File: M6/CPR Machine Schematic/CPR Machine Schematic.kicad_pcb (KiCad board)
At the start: 2 copper layers, 134 x 94 mm, 67 parts, among them J1 Contactor 22.2V IN, J10 Stop Button Port, J11 Go Button Port, J12 I2C Port, J13 Raspberry_Pi_2_3, J2 5V Spare Headers, J3 Power Switch, J4 3V3 Spare Headers, J5 12 Spare headers, J6 Battery Spare headers, J7 GND Spare Headers, J8 Force Sensor, J9 Laser Port, Q1 2N3904, Q2 DMG2305UX-13 MOSFET, Q3 FDMS8350LET40, Q4 DMMT5401 PNP, Q6 FDMS8350LET40, Q7 FDMS8350LET40, U1 LT1765EFE-5_PBF, U2 MAX42402AFLB+, U3 MCP6001R, U4 12V Buck, U6 3.3V Buck

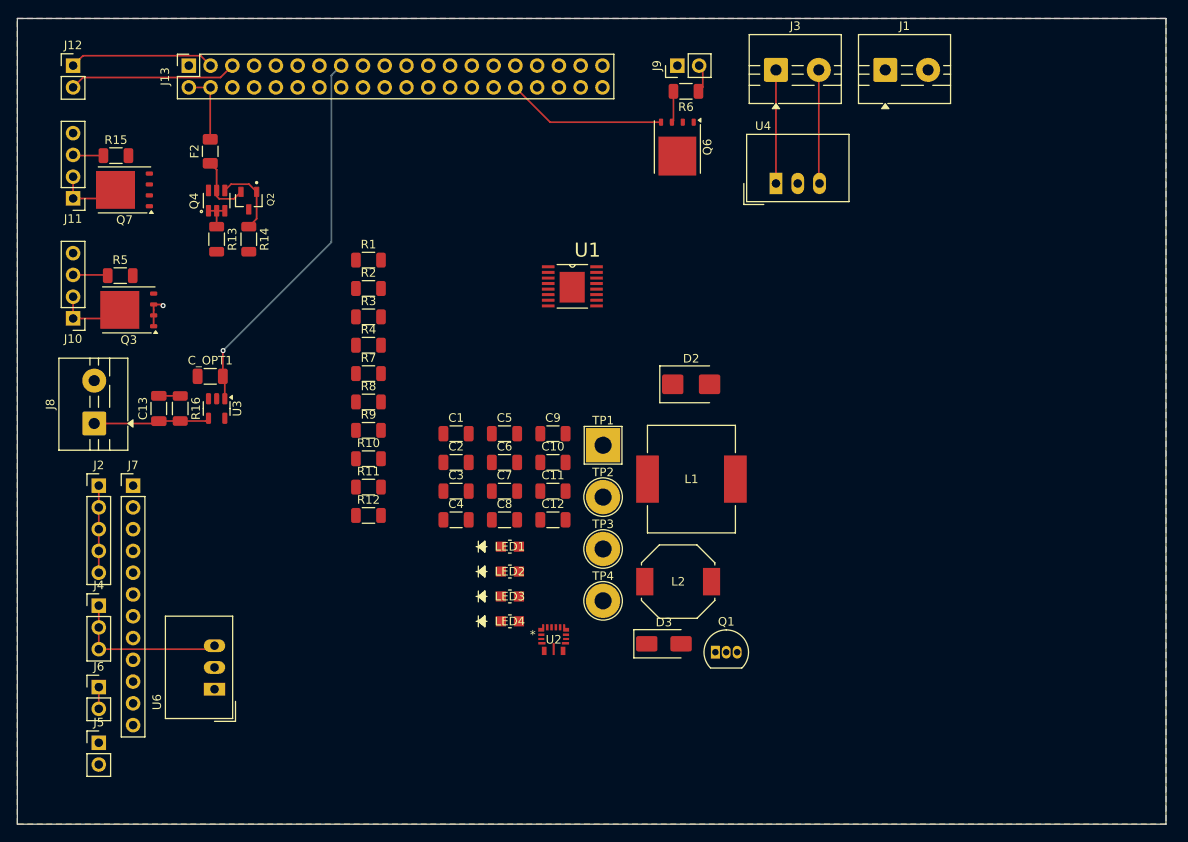
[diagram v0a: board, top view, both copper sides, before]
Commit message: finished PCB Draft
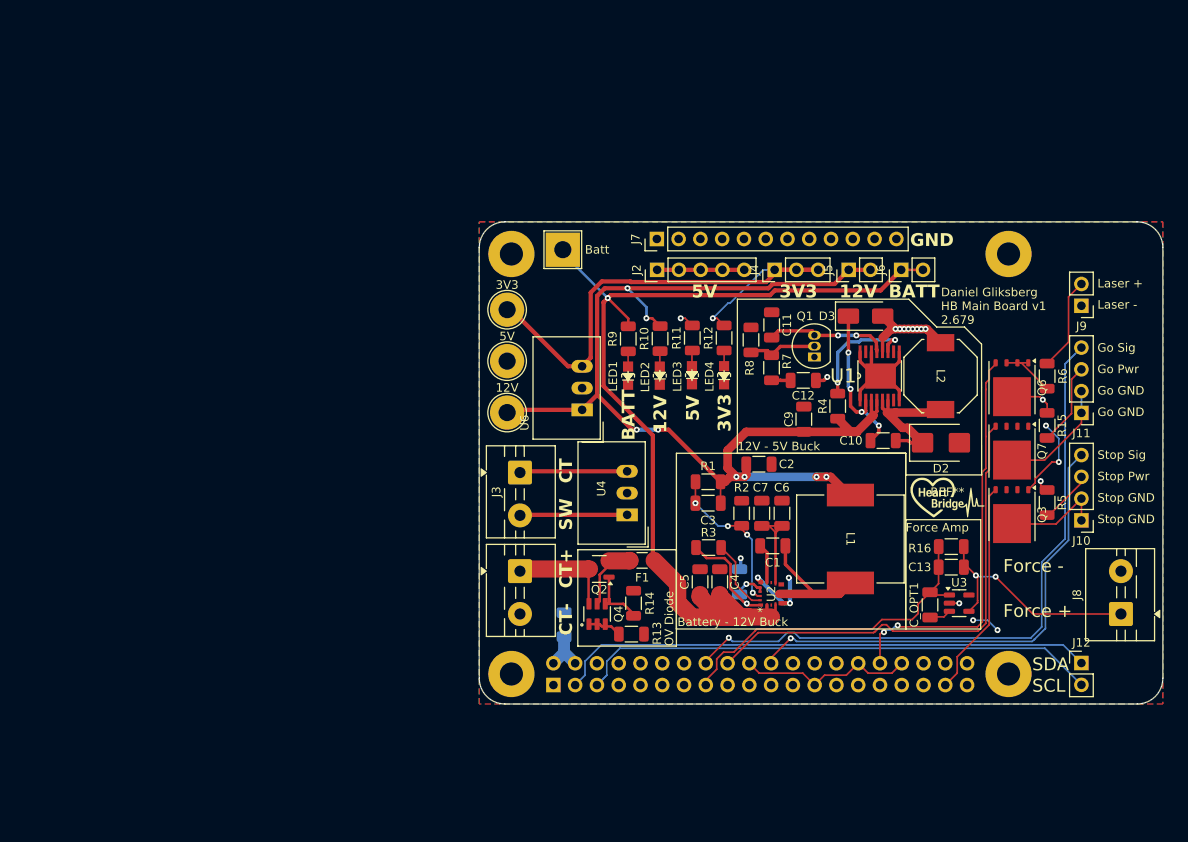
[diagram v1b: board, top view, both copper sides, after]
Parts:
- added F1: 5A, Fuse:Fuse_1206_3216Metric, F.Cu at (133.9, 111.7)
- added REF**: MountingHole_2.7mm_Pad, MountingHole:MountingHole_2.7mm_Pad, F.Cu at (118.6, 76.0)
- added REF**: MountingHole_2.7mm_Pad, MountingHole:MountingHole_2.7mm_Pad, F.Cu at (176.6, 125.0)
- added REF**: Untitled, MAX42402AFLB_:Untitled, F.Cu at (169.5, 104.2)
- added REF**: MountingHole_2.7mm_Pad, MountingHole:MountingHole_2.7mm_Pad, F.Cu at (118.6, 125.0)
- added REF**: MountingHole_2.7mm_Pad, MountingHole:MountingHole_2.7mm_Pad, F.Cu at (176.6, 76.0)
- C8, J13: moved to B.Cu
- F2: value 4A -> 3A; moved to B.Cu
- Q2: value DMG2305UX-13 MOSFET -> AO3407A; footprint 2679:SOT91P240X110-3N -> Package_TO_SOT_SMD:SOT-23-3
- moved J12 136.7 mm to (185.1, 123.7)
- moved J8 121.8 mm to (189.8, 118.0)
- moved J11 120.3 mm to (185.1, 94.5)
- moved J10 120.0 mm to (185.1, 107.1)
- moved R15 113.1 mm to (181.1, 96.0), turned to 90 degrees
- moved R5 111.3 mm to (181.1, 105.0), turned to 90 degrees
- moved Q7 107.9 mm to (177.0, 99.0), turned to -90 degrees
- moved Q3 105.8 mm to (177.0, 106.4), turned to -90 degrees
- moved J6 105.5 mm to (164.1, 77.8), turned to 90 degrees
- moved J5 103.4 mm to (158.0, 77.8), turned to 90 degrees
- moved C13 94.3 mm to (169.9, 112.5), turned to 180 degrees
- moved R16 91.4 mm to (169.9, 110.1), turned to 0 degrees
- moved U3 89.6 mm to (170.9, 116.7), turned to 0 degrees
- moved C_OPT1 88.1 mm to (167.5, 116.9), turned to 90 degrees
- moved J4 88.0 mm to (149.3, 77.8), turned to 90 degrees
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- renumbered TP2 to 12V, TP4 to 3V3, TP3 to 5V, TP1 to Batt
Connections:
- net /HMI_Raspi/Go_Button renamed /HMI_Raspi/Go Button
- net /HMI_Raspi/Stop_Button renamed /HMI_Raspi/Stop Button
- net Net-(J10-Pin_1) renamed /HMI_Raspi/Stop Button Ground
- net Net-(J10-Pin_3) renamed /HMI_Raspi/Stop LED Power
- net Net-(J11-Pin_1) renamed /HMI_Raspi/Go Button Ground
- net Net-(J11-Pin_3) renamed /HMI_Raspi/Go LED Power
- C8 pad 1: Net-(U2-GND) -> GND
- F2 pad 1: Net-(F2-Pad1) -> +5V
- J1 pad 1: +22.2V -> /Power/Contactor +
- J3 pad 1: Net-(J3-Pin_1) -> /Power/To Contactor
- J3 pad 2: Net-(J3-Pin_2) -> /Power/From Switch
- Q2 pad 2: Net-(F2-Pad1) -> Net-(F1-Pad1)
- Q2 pad 3: +5V -> /Power/Contactor +
- Q4 pad 5: Net-(F2-Pad1) -> Net-(F1-Pad1)
- Q4 pad 6: +5V -> /Power/Contactor +
- U2 pad 11: Net-(C6-Pad2) -> Net-(U2-BIAS)
- U2 pad 12: unconnected-(U2-NC-Pad12) -> Net-(U2-BIAS)
- U2 pad 13: Net-(U2-BST) -> Net-(U2-FB)
- U2 pad 14: Net-(U2-GND) -> Net-(U2-PGOOD)
- U2 pad 8: GND -> unconnected-(U2-NC-Pad8)
- U2 pad 9: Net-(U2-LX) -> Net-(U2-BST)
- U4 pad 1: Net-(J3-Pin_1) -> /Power/From Switch
- U4 pad 3: Net-(J3-Pin_2) -> /Power/To Contactor
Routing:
- net +12V: track 0.00 -> 132.3 mm, vias 0 -> 8
- net +22.2V: track 2.54 -> 114.6 mm, vias 0 -> 1
- net /HMI_Raspi/Go Button: track 0.00 -> 76.5 mm, vias 0 -> 1
- net GND: track 3.70 -> 67.6 mm, vias 1 -> 8
- net /HMI_Raspi/Stop Button: track 0.00 -> 56.3 mm, vias 0 -> 1
- net /HMI_Raspi/Go_Enable: track 0.00 -> 56.2 mm
- net /Raspi/I2C_SDA: track 17.0 -> 62.8 mm
- net +3.3V: track 18.7 -> 64.5 mm, vias 0 -> 1
- net /Raspi/I2C_SCL: track 19.6 -> 61.0 mm
- net /HMI_Raspi/Laser_PWM: track 18.7 -> 47.1 mm, vias 0 -> 2
- net /HMI_Raspi/Stop_Enable: track 0.00 -> 25.2 mm
- net +5V: track 10.2 -> 33.0 mm, vias 0 -> 13
- net Net-(D3-K): track 0.00 -> 18.8 mm, vias 0 -> 4
- net Net-(D2-K): track 0.00 -> 18.4 mm
- net Net-(U2-FB): track 0.00 -> 18.4 mm, vias 0 -> 4
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- added copper zone on B.Cu, net +5V
- added copper zone on F.Cu, net GND
- removed copper zone on F.Cu, net +5V
- removed copper zone on B.Cu, net GND
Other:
- board size 134 x 94 mm -> 79.8 x 56.2 mm
- board text added: "12V"
- board text added: "12V - 5V Buck"
- board text added: "3V3"
- board text added: "5V"
- board text added: "BATT"
- board text added: "Battery - 12V Buck"
- board text added: "CT"
- board text added: "CT+"
- board text added: "CT-"
- board text added: "Daniel Gliksberg HB Main Board v1 2.679"
- board text added: "Force +"
- board text added: "Force -"
- board text added: "Force Amp"
- board text added: "GND"
- board text added: "Go GND"
- board text added: "Go Pwr"
- board text added: "Go Sig"
- board text added: "Laser +"
- board text added: "Laser -"
- board text added: "OV Diode"
- board text added: "SCL"
- board text added: "SDA"
- board text added: "SW"
- board text added: "Stop GND"
- board text added: "Stop Pwr"
- board text added: "Stop Sig"
